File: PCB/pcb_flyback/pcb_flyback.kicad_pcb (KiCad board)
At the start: 2 copper layers, 43 parts, among them Q1 IRF540N, U1 TL494, U2 PC817

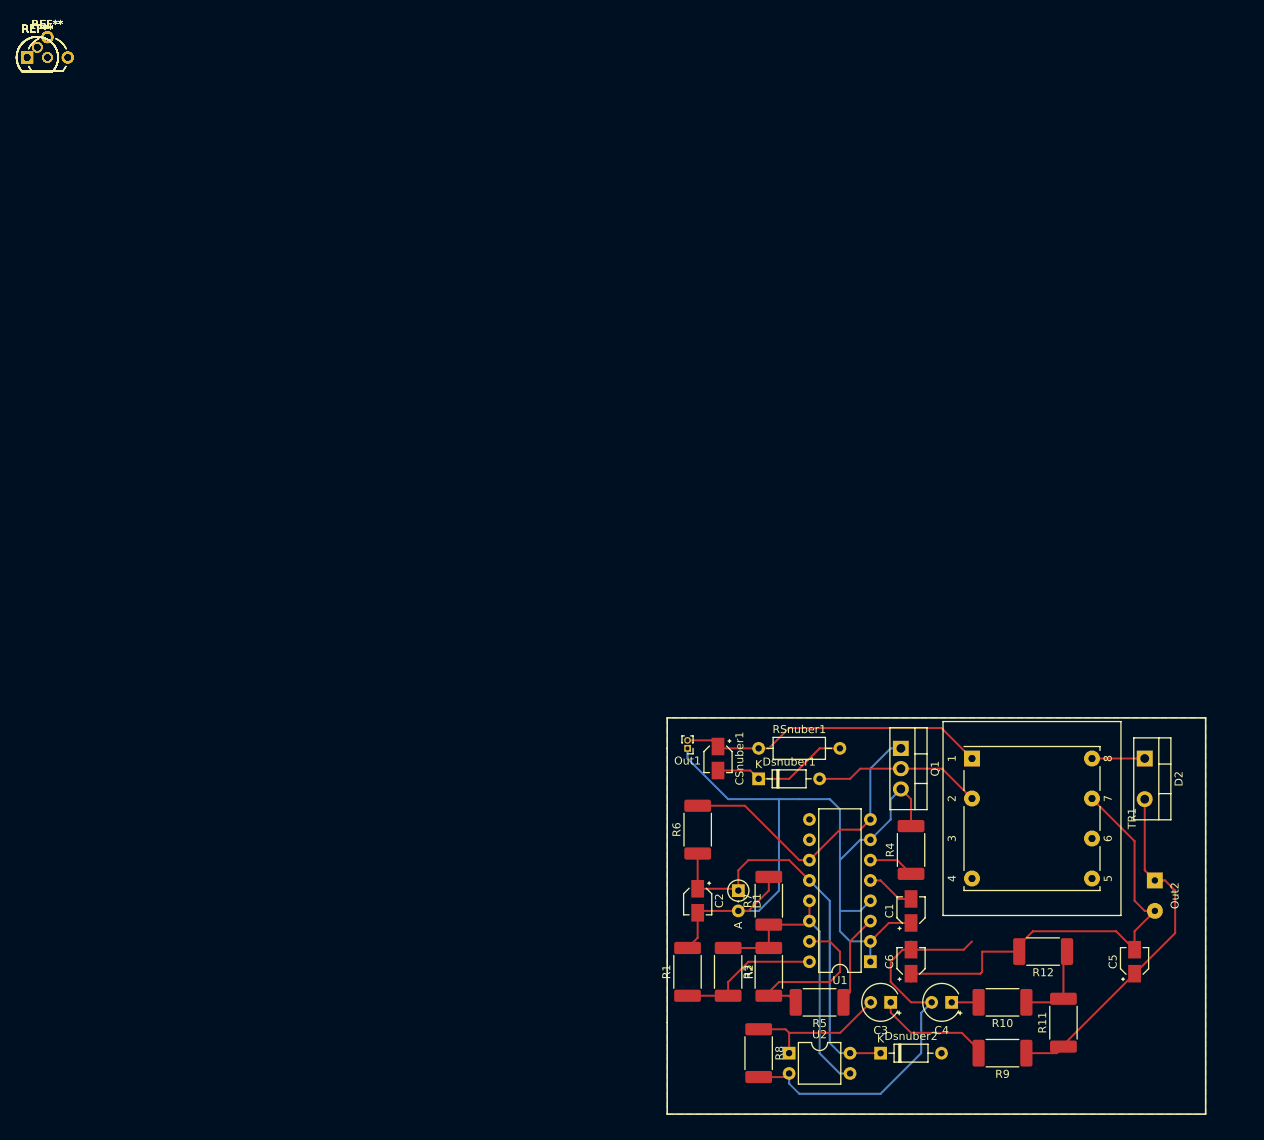
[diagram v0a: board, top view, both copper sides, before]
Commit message: PCB 99% listo
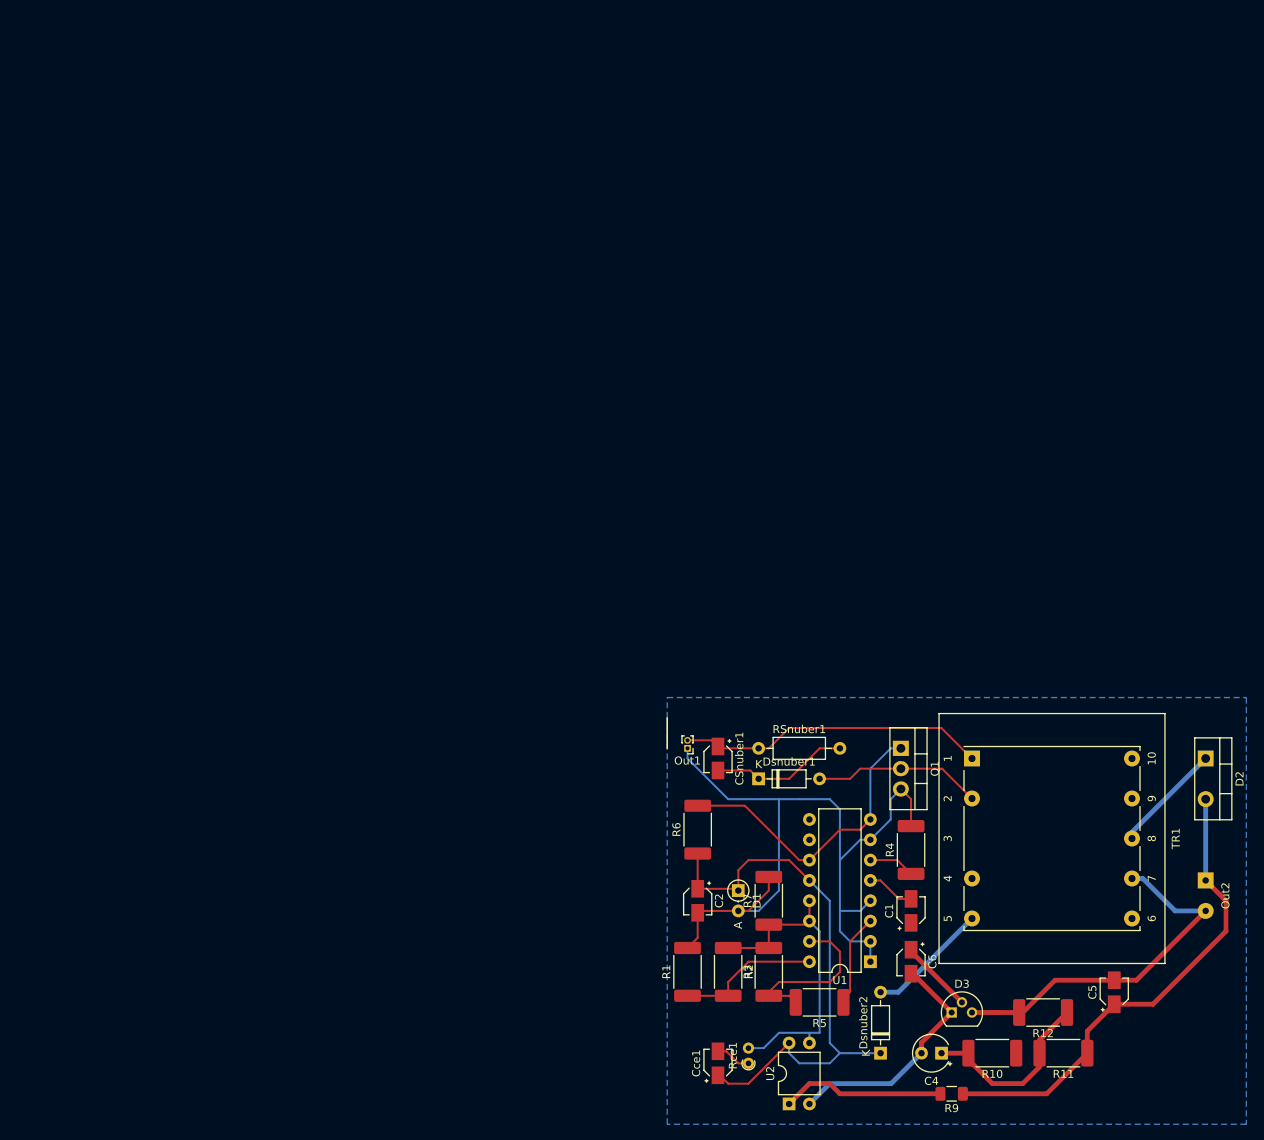
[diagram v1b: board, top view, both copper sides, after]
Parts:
- removed C3: C, Capacitor_THT:CP_Radial_Tantal_D4.5mm_P2.50mm
- removed R8: R, Resistor_SMD:R_2512_6332Metric_Pad1.52x3.35mm_HandSolder
- removed REF** (x3): TO-92L_Wide, Package_TO_SOT_THT:TO-92L_Wide
- removed REF** (x6): TO-92, Package_TO_SOT_THT:TO-92
- removed REF** (x4): TO-92L, Package_TO_SOT_THT:TO-92L
- added Cce1: 1m, Capacitor_SMD:CP_Elec_3x5.3, F.Cu at (86.4, 125.7)
- added D3: TL431D, Package_TO_SOT_THT:TO-92L, F.Cu at (115.6, 119.4)
- added Rce1: 8k, Resistor_THT:R_Axial_DIN0204_L3.6mm_D1.6mm_P1.90mm_Vertical, F.Cu at (90.2, 125.7)
- C1: value C -> 1n
- C2, C4: value C -> 22n
- C5: value C -> 500u
- C6: value C -> 1u
- CSnuber1: value C -> 55.2u
- D1: value D_Zener -> 15V
- D2: value DIODE -> RFU10TF6S
- R1, R2: value R -> 51k
- R10: value R -> 1m
- R11: value R -> 38k
- R12, R4: value R -> 10k
- R3: value R -> 510
- R5: value R -> 5.1k
- R6: value R -> 150
- R7: value R -> 860
- R9: value R -> 4.2k; footprint Resistor_SMD:R_2512_6332Metric_Pad1.52x3.35mm_HandSolder -> Resistor_SMD:R_1206_3216Metric
- RSnuber1: value R -> 4k
- TR1: footprint Transformer_THT:Transformer_Breve_TEZ-22x24 -> Transformer_THT:Transformer_Breve_TEZ-28x33
- moved R9 8.13 mm to (115.6, 129.5)
- moved D2 7.62 mm to (147.3, 87.6)
- moved R12 7.62 mm to (127.0, 119.4)
- moved C4 6.48 mm to (114.3, 124.5)
- moved R10 6.48 mm to (120.7, 124.5)
- moved U2 6.35 mm to (95.2, 130.8), turned to 90 degrees
- moved Out2 6.35 mm to (147.3, 102.9)
- moved C5 4.58 mm to (135.9, 116.8)
- moved R11 3.81 mm to (129.5, 124.5), turned to 180 degrees
- turned C6 to 270 degrees
- turned Dsnuber2 to 90 degrees
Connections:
- R11 pad 2: Net-(D3-Pad8) -> Net-(C4-Pad1)
- R12 pad 1: Net-(D3-Pad8) -> Net-(C4-Pad1)
- R9 pad 2: Net-(C3-Pad1) -> Net-(R9-Pad2)
- U2 pad 1: Net-(C3-Pad2) -> Net-(R9-Pad2)
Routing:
- net Net-(C4-Pad2): track 52.3 -> 31.7 mm
- net Net-(R9-Pad2): track 0.00 -> 20.5 mm
- net Net-(C2-Pad1): track 50.8 -> 70.9 mm
- net Net-(C4-Pad1): track 3.36 -> 23.4 mm
- net Net-(C3-Pad2): track 18.3 -> 0.00 mm
- net Net-(C5-Pad1): track 44.0 -> 60.5 mm
- net Net-(Dsnuber2-Pad2): track 0.00 -> 15.2 mm
- net Net-(C3-Pad1): track 14.6 -> 0.00 mm
- net Net-(D3-Pad8): track 10.9 -> 0.00 mm
- net Net-(D2-Pad1): track 6.59 -> 13.8 mm
- net GND: track 107.6 -> 101.6 mm
- net Net-(Cce1-Pad2): track 0.00 -> 4.43 mm
- net Net-(R2-Pad1): track 37.7 -> 41.2 mm
- net Net-(C5-Pad2): track 58.6 -> 59.7 mm
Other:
- net class Default: trace_width 0.25 -> 0.6
